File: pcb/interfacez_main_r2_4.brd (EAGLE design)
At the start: 86 x 58 mm, 172 parts, among them IC1 STMPS2141STR, IC10 74LCX245FT, IC11 74LCX245FT, IC12 USB1T11AMTCX, IC13 74LVC06APW,118, IC2 EP4CE6E22C8N, IC3 74LCX245FT, IC4 74LCX245FT, IC5 MP2233DJ, IC6 MP2233DJ, IC7 CH330N, IC8 MIC5504-2.5YM5-TR, IC9 LY68L6400SLIT, J1 AMPHENOL_ICC_-_FCI_20021121-0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, J2 503398-1892, Q1 BSS123, Q2 BSS138DW, Q3 BSS123, Q4 BSS84DW, Q5 BSS84DW, Q6 BSS84DW, T2 DMP2240UDM, U1 ESP-WROOM-32

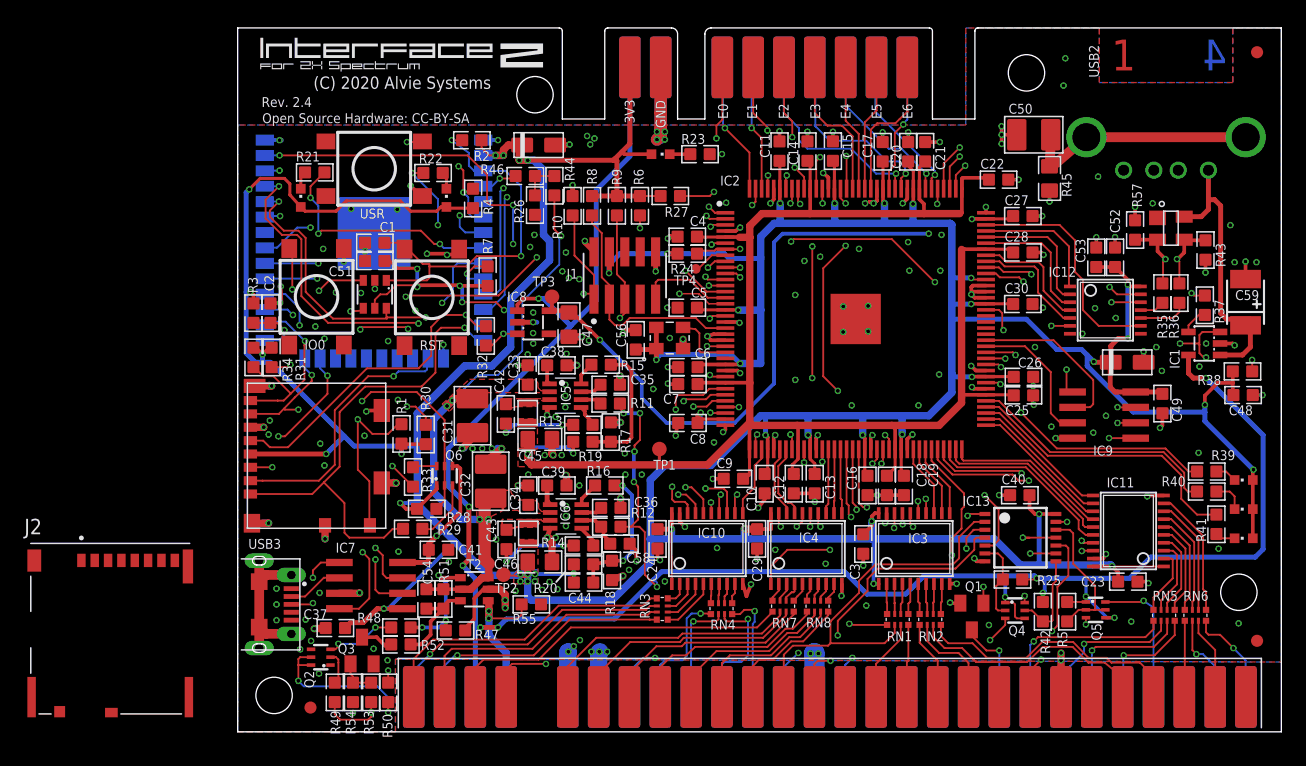
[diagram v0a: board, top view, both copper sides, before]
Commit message: Add r2.4 mainboard files
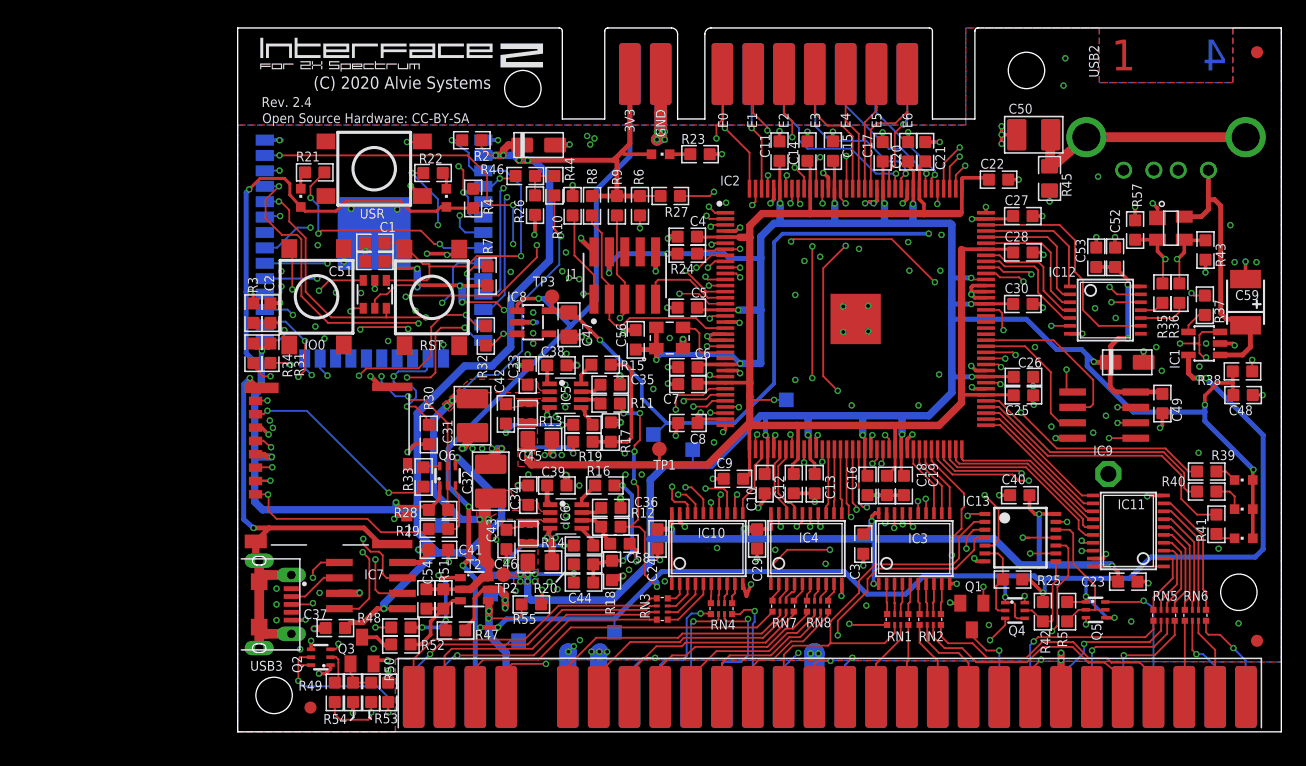
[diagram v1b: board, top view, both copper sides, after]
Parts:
- removed R1: 10K, GadgetFactory:0603
- removed SD1: 1040310811, alvie:1040310811
- added T+12V, T+1V2, T+2V5, T+3V3, T+5V, T+9V, TP5: TPTP12SQ, testpad:TP12SQ
- TP4: value TPTP08R -> TPPAD1-13; device testpad:TP08R -> testpad:P1-13
- moved TP4 38.0 mm to (71.8, 21.2)
- moved J2 22.2 mm to (7.10, 21.9), turned to 90 degrees
- moved R29 2.12 mm to (16.6, 16.7)
- moved R28 0.98 mm to (16.6, 18.3)
- moved R33 0.88 mm to (15.3, 21.0)
- moved U$5 0.55 mm to (43.8, 54.2)
- moved R31 0.36 mm to (2.70, 31.2)
- moved R34 0.35 mm to (1.30, 31.2)
- moved Q6 0.25 mm to (17.3, 21.1)
- moved R30 0.25 mm to (15.8, 24.5)
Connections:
- removed net N$1: IC2.8, TP4.TP
- removed net SDMMC_DET: R1.2, SD1.A, U1.28
- removed net VDD: J2.4
- removed net VSS: J2.6, J2.9
- new net IO6: IC2.8, U1.28
- net +12V: now also T+12V.TP
- net +1V2: now also T+1V2.TP
- net +2V5: now also T+2V5.TP
- net +3V3: now also J2.4, T+3V3.TP; no longer R1.1, SD1.4
- net +5V: now also T+5V.TP
- net +9V: now also T+9V.TP
- net GND: now also J2.6, J2.9, TP4.TP; no longer SD1.6, SD1.B, SD1.MNT1, SD1.MNT2, SD1.MNT3, SD1.MNT4
- net PE: now also J2.P1, J2.P2, J2.P3, J2.P4
- net SDMMC_CK: now also J2.5; no longer SD1.5
- net SDMMC_CMD: now also J2.3; no longer SD1.3
- net SDMMC_D0: now also J2.7; no longer SD1.7
- net SDMMC_D1: now also J2.8; no longer SD1.8
- net SDMMC_D2: now also J2.1; no longer SD1.1
- net SDMMC_D3: now also J2.2; no longer SD1.2
- net VSWITCH: now also TP5.TP
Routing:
- net PE: track 172.1 -> 217.1 mm, vias 0 -> 3
- net IO6: track 0.00 -> 44.4 mm, vias 0 -> 2
- net SDMMC_DET: track 28.2 -> 0.00 mm, vias 2 -> 0
- net +3V3: track 541.5 -> 551.3 mm, vias 52 -> 53
- net GND: track 166.7 -> 175.1 mm, vias 236 -> 227
- net PULLUP_EN: track 33.9 -> 30.3 mm, vias 2 -> 3
- net +1V2: track 141.4 -> 144.5 mm, vias 2 -> 3
- net N$1: track 2.90 -> 0.00 mm
- net SDMMC_D0: track 21.6 -> 24.3 mm
- net SDMMC_D2: track 40.0 -> 42.3 mm, vias 1 -> 3
- net +5V: track 200.8 -> 202.9 mm
- net +9V: track 34.6 -> 36.2 mm
- net VSWITCH: track 50.3 -> 51.9 mm
- net +2V5: track 62.4 -> 63.9 mm
- net ESP_RX: track 49.1 -> 47.7 mm
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
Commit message: pcb: fix R44 value for voltage divider
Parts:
- R44: value 30K1 1% -> 39K1 1%
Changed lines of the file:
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@@
 <grid distance="0.25" unitdist="mm" unit="mm" style="lines" multiple="1" display="yes" altdistance="0.05" altunitdist="mm" altunit="mm"/>
 <layers>
-<layer number="1" name="Top" color="4" fill="1" visible="no" active="yes"/>
+<layer number="1" name="Top" color="4" fill="1" visible="yes" active="yes"/>
 <layer number="2" name="GND" color="11" fill="3" visible="no" active="yes"/>
 <layer number="3" name="Route3" color="4" fill="3" visible="no" active="no"/>
 <layer number="14" name="Route14" color="1" fill="6" visible="no" active="no"/>
 <layer number="15" name="Route" color="13" fill="1" visible="no" active="yes"/>
-<layer number="16" name="PWR" color="1" fill="1" visible="no" active="yes"/>
-<layer number="17" name="Pads" color="2" fill="1" visible="no" active="yes"/>
-<layer number="18" name="Vias" color="2" fill="1" visible="no" active="yes"/>
+<layer number="16" name="PWR" color="1" fill="1" visible="yes" active="yes"/>
+<layer number="17" name="Pads" color="2" fill="1" visible="yes" active="yes"/>
+<layer number="18" name="Vias" color="2" fill="1" visible="yes" active="yes"/>
 <layer number="19" name="Unrouted" color="6" fill="1" visible="no" active="yes"/>
 <layer number="20" name="Dimension" color="15" fill="1" visible="yes" active="yes"/>
@@
 <attribute name="VALUE" x="25.05" y="44.8" size="0.05" layer="27" font="vector" ratio="0" rot="R270"/>
 </element>
-<element name="R44" library="GadgetFactory" package="0603" value="30K1 1%" x="26.1" y="45" smashed="yes" rot="R270">
+<element name="R44" library="GadgetFactory" package="0603" value="39K1 1%" x="26.1" y="45" smashed="yes" rot="R270">
 <attribute name="NAME" x="26.95" y="47.35" size="0.8128" layer="25" ratio="16" rot="R270"/>
 <attribute name="VALUE" x="26.65" y="46.4" size="0.05" layer="27" font="vector" ratio="0" rot="R270"/>
@@
 </signal>
 </signals>
-<errors>
-</errors>
 </board>
 </drawing>
